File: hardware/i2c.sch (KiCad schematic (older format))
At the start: 0 parts

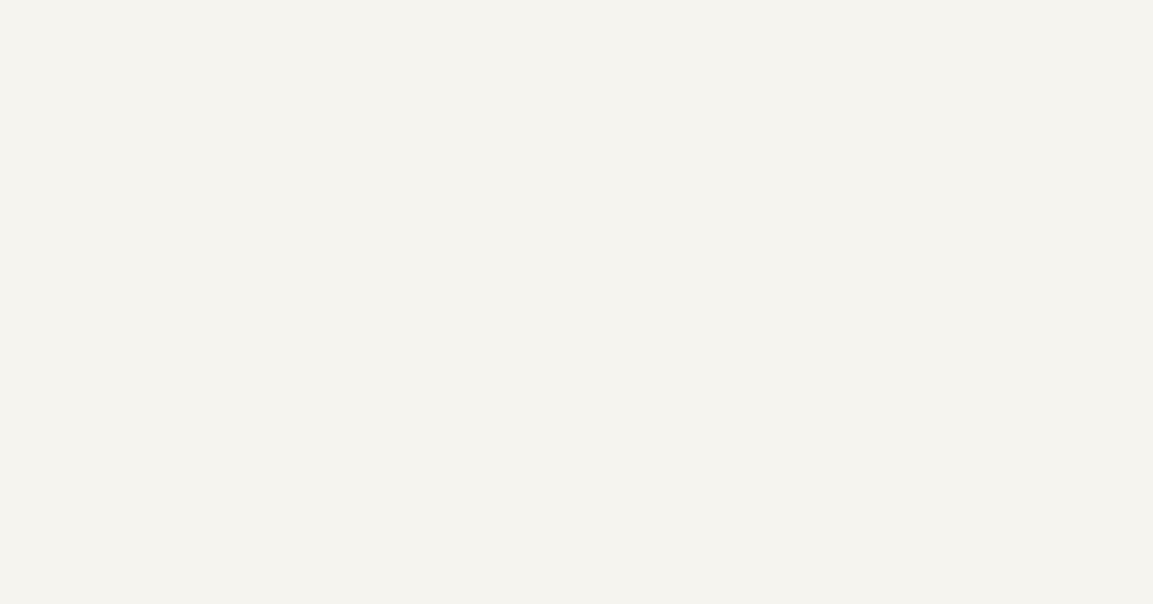
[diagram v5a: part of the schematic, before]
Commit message: update,
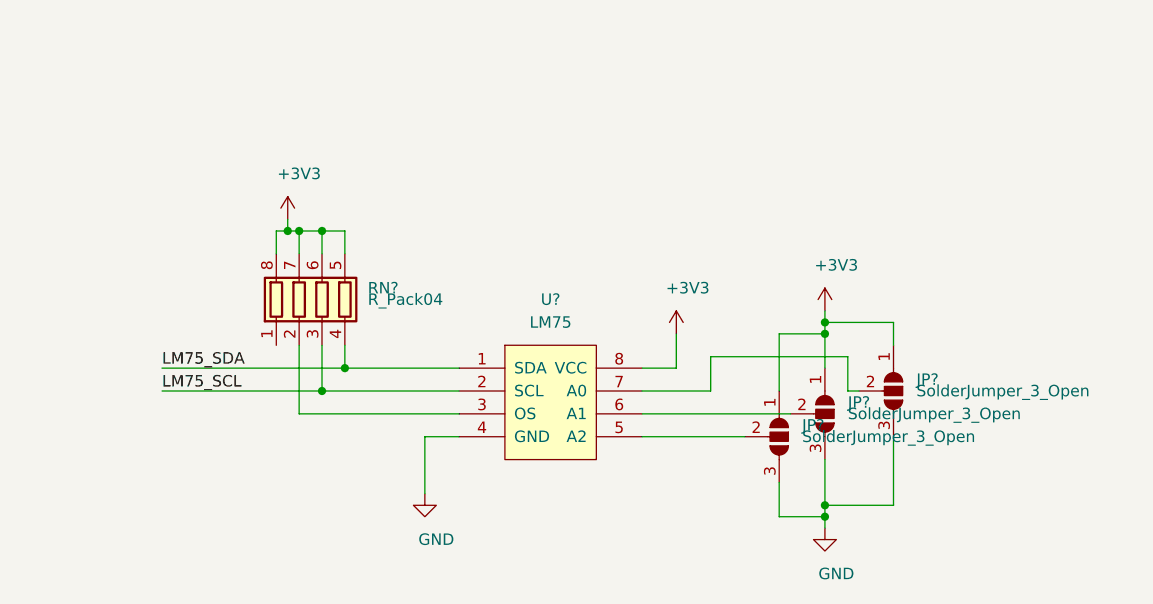
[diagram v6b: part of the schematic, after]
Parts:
- added JP? (x3): SolderJumper_3_Open, symbol Jumper:SolderJumper_3_Open
- added RN?: R_Pack04, symbol Device:R_Pack04
- added U?: LM75, Package_SO:SOP-8_3.76x4.96mm_P1.27mm, symbol taobao-components:LM75
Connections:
- new net: RN?.2 (R2.1), U?.3 (OS)
- new net: JP?.2 (C), U?.5 (A2)
- new net: JP?.2 (C), U?.6 (A1)
- new net: JP?.2 (C), U?.7 (A0)
- new net +3V3: JP?.1 (A), JP?.1 (A), JP?.1 (A), RN?.5 (R4.2), RN?.6 (R3.2), RN?.7 (R2.2), RN?.8 (R1.2), U?.8 (VCC)
- new net GND: JP?.3 (B), JP?.3 (B), JP?.3 (B), U?.4 (GND)
- new net LM75_SCL: RN?.3 (R3.1), U?.2 (SCL)
- new net LM75_SDA: RN?.4 (R4.1), U?.1 (SDA)
